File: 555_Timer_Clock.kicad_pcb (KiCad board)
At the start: 2 copper layers, 39 x 25 mm, 17 parts, among them J1 +5V, J2 CLK_Out, SW1 Trigger, SW2 RST, U1 ICM7555xB

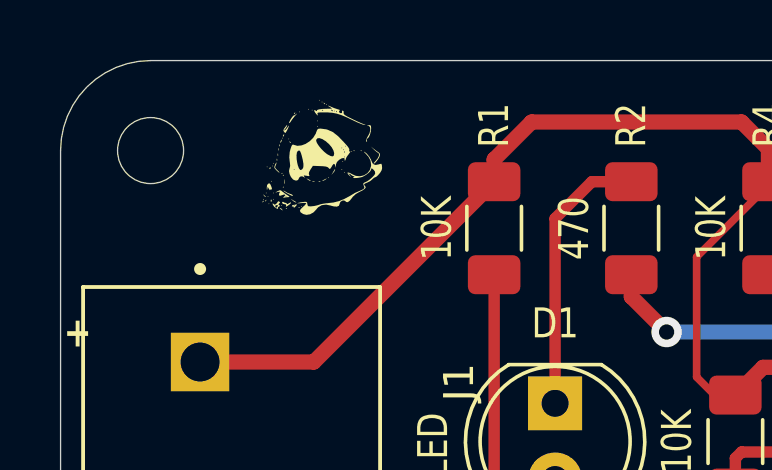
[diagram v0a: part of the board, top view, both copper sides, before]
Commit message: Update
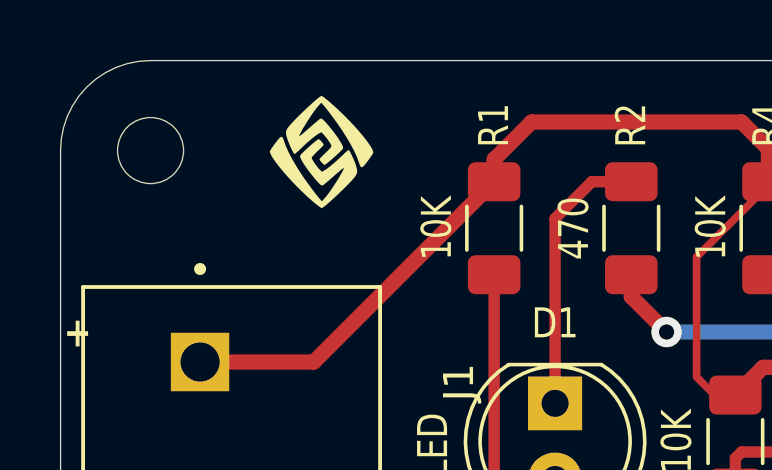
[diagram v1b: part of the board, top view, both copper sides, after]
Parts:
- removed the G*** at (105.5, 63.5)
- added G***: LOGO, my_footprints:geo, F.Cu at (105.5, 63.5)
